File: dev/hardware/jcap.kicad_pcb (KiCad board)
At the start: 2 copper layers, 136.8 x 87 mm, 66 parts, among them J201 CPU PGMR, J202 SPARE CPU HDR, J203 GPU PGMR, J204 SPARE GPU HDR, J301 DC IN, J501 VGA OUT, J601 CONTROLS, Q301 IPP80P03P4L-04, SW201 CPU ~{RES}, SW202 DEBUG, SW203 GPU ~{RES}, SW601 TILT, U201 P8X32A-D40, U202 P8X32A-D40, U301 LF33_TO220, U401 24LC256, U402 24LC256, U601 74HC165, U602 74HC165, Y201 6.5MHz, Y202 6.5MHz

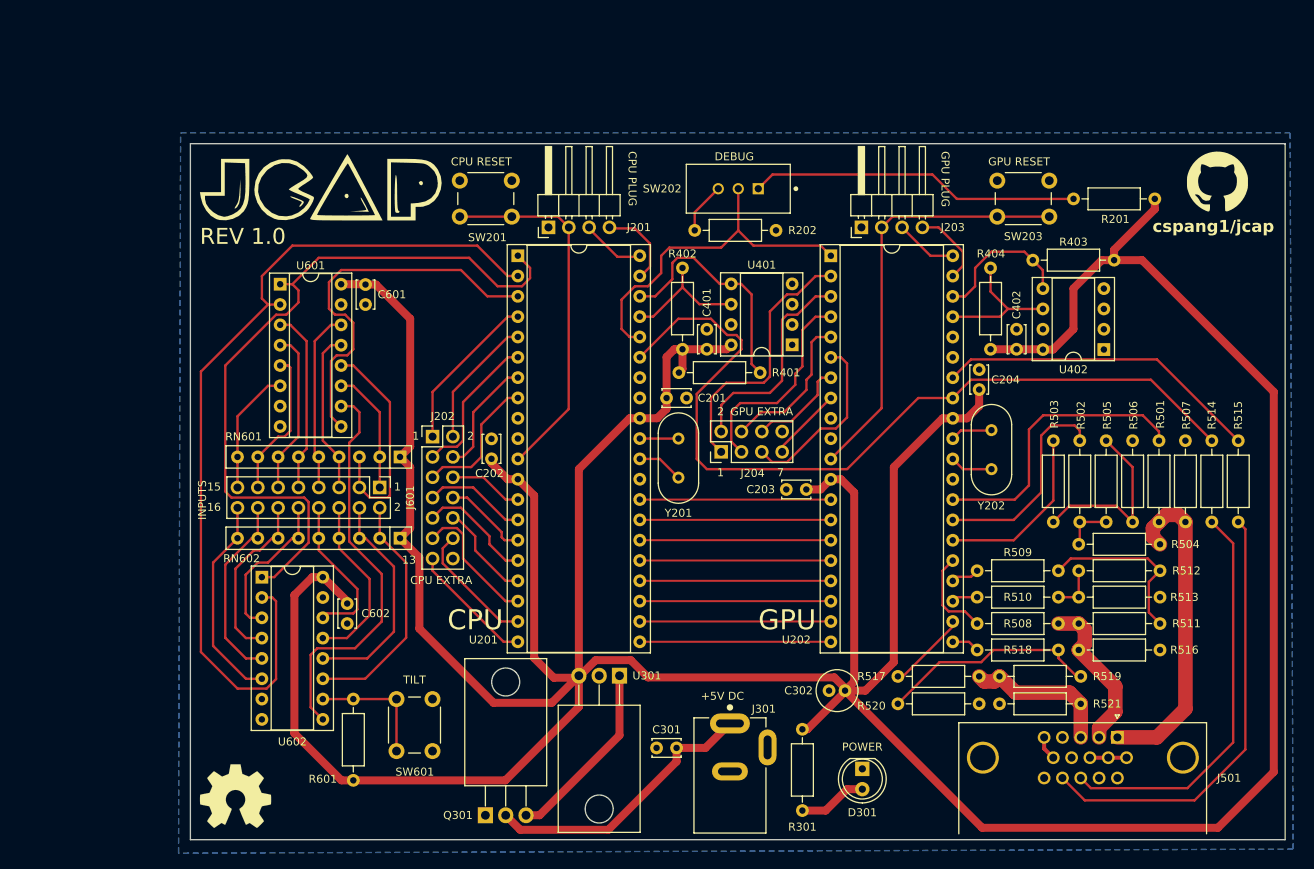
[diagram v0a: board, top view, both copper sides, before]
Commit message: Finalized dev board administrivia
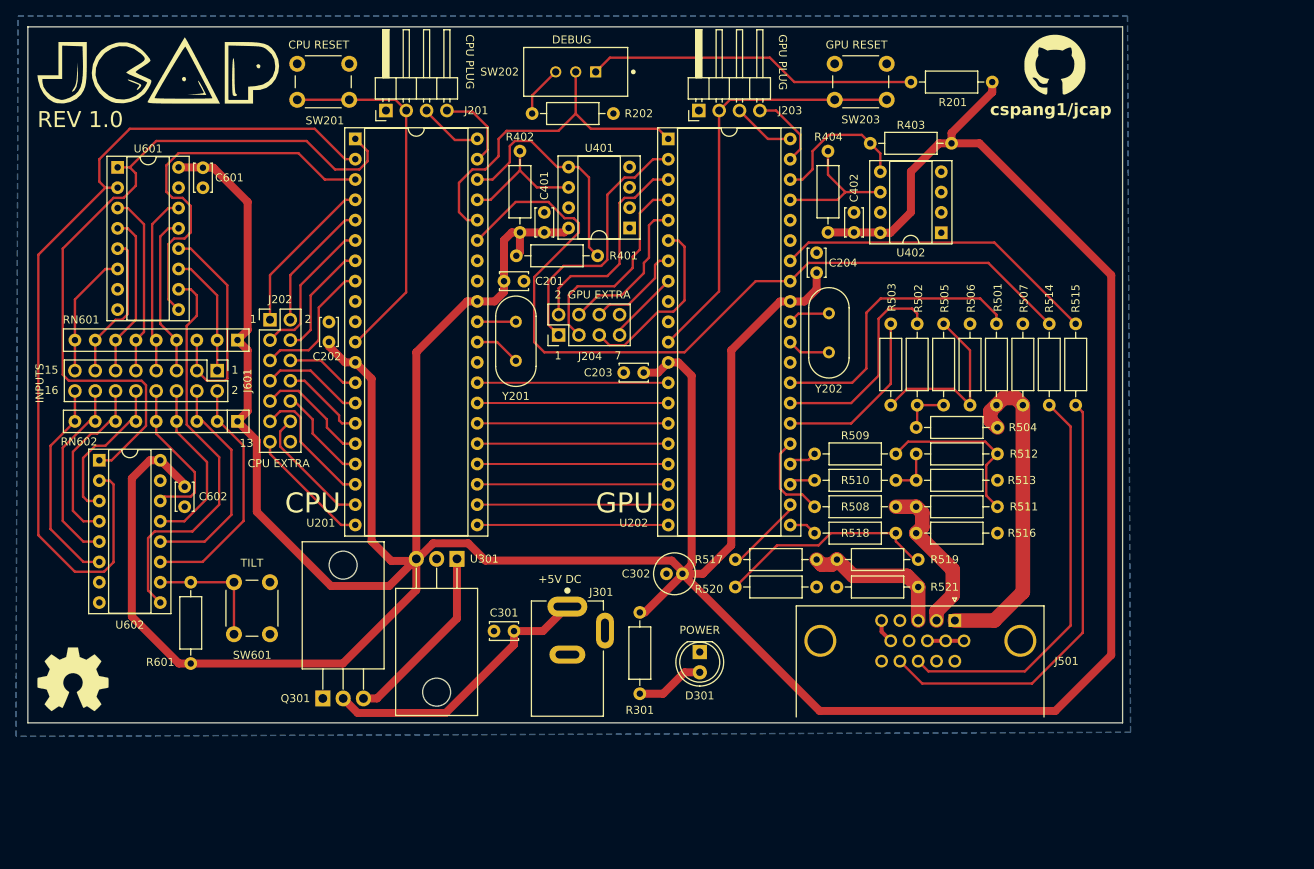
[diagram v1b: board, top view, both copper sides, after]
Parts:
- R201, R202: value 200 -> 10K
- U201, U202: value P8X32A-D40 -> P8X32A
- U301: value LF33_TO220 -> LM3940IT
- moved R202 33.8 mm to (140.7, 62.2), turned to 0 degrees
- moved R515 32.0 mm to (208.7, 88.5), turned to -90 degrees
- moved D301 25.0 mm to (161.7, 129.5)
- moved C201 25.0 mm to (139.7, 83.2)
- moved J204 25.0 mm to (144.0, 89.9)
- moved R401 25.0 mm to (148.9, 80.0)
- moved R502 25.0 mm to (188.8, 98.7)
- moved R510 25.0 mm to (186.2, 108.1)
- moved R518 25.0 mm to (186.2, 114.7)
- moved SW203 25.0 mm to (178.5, 56.0)
- moved REF** 25.0 mm to (83.3, 133.0)
- moved J201 25.0 mm to (122.4, 61.9)
- moved J202 25.0 mm to (108.0, 88.0)
- moved R507 25.0 mm to (202.1, 88.5)
- moved R508 25.0 mm to (186.2, 111.4)
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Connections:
- R202 pad 1: GND -> Net-(R202-Pad1)
- R202 pad 2: Net-(R202-Pad2) -> GND
- R515 pad 1: Net-(J501-Pad14) -> H_SYNC
- R515 pad 2: H_SYNC -> Net-(J501-Pad14)
- SW202 pad 3: Net-(R202-Pad2) -> Net-(R202-Pad1)
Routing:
- net Net-(R202-Pad2): track 6.43 -> 0.00 mm
- net Net-(R202-Pad1): track 0.00 -> 6.43 mm
